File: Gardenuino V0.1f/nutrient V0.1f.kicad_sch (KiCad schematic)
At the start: 84 parts, among them J1 Conn_01x04_Male, J2 Conn_01x04_Female, J3 Conn_01x04_Male, J4 Conn_01x04_Male, J5 Conn_01x04_Female, J6 Conn_01x04_Male, J7 Conn_01x03_Male, J8 Conn_01x03_Male, P1 SolderJumper_2_Open, P2 SolderJumper_2_Bridged, P3 SolderJumper_2_Bridged, Q1 Q_NMOS_DGS, Q10 Q_NMOS_DGS, Q2 Q_NMOS_DGS, Q3 Q_NMOS_DGS, Q4 Q_NMOS_DGS, Q5 Q_NMOS_DGS, Q6 Q_NMOS_DGS, Q7 Q_NMOS_DGS, Q8 2N3904, U1 23LC512, U2 DS1307+, Y1 Crystal_Small

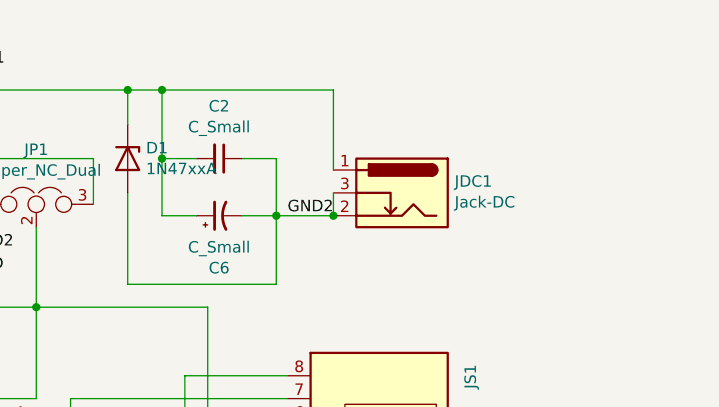
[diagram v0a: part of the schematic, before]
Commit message: SpectDrone development
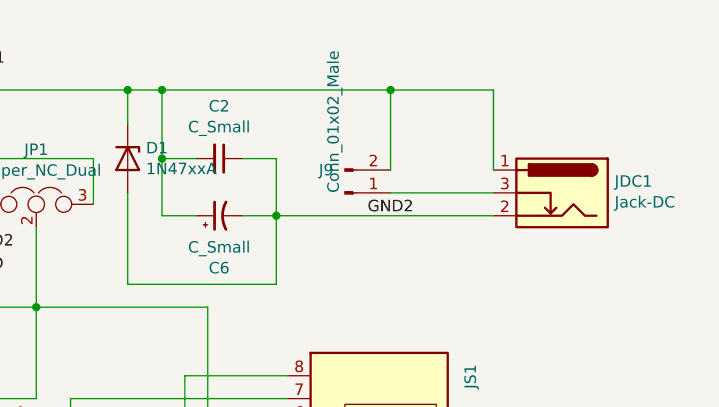
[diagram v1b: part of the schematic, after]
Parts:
- added J9: Conn_01x02_Male, Connector_PinHeader_2.54mm:PinHeader_1x02_P2.54mm_Vertical, symbol Connector:Conn_01x02_Male
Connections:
- net GND: no longer JDC1.3
- net VIN1: now also J9.2 (Pin_2)
- new net: J9.1 (Pin_1), JDC1.3
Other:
- moved on the sheet: JDC1
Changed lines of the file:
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@@
   (junction (at 267.97 110.49) (diameter 0) (color 0 0 0 0)
   )
+  (junction (at 250.19 17.78) (diameter 0) (color 0 0 0 0)
+  )
   (junction (at 227.33 125.73) (diameter 0) (color 0 0 0 0)
   )
@@
   )
   (junction (at 68.58 115.57) (diameter 0) (color 0 0 0 0)
-  )
-  (junction (at 243.84 31.75) (diameter 0) (color 0 0 0 0)
   )
   (junction (at 83.82 113.03) (diameter 0) (color 0 0 0 0)
@@
     (stroke (width 0) (type default) (color 0 0 0 0))
   )
+  (wire (pts (xy 237.49 31.75) (xy 261.62 31.75))
+    (stroke (width 0) (type default) (color 0 0 0 0))
+  )
   (wire (pts (xy 104.14 157.48) (xy 134.62 157.48))
     (stroke (width 0) (type default) (color 0 0 0 0))
@@
     (stroke (width 0) (type default) (color 0 0 0 0))
   )
-  (wire (pts (xy 243.84 31.75) (xy 237.49 31.75))
-    (stroke (width 0) (type default) (color 0 0 0 0))
-  )
   (wire (pts (xy 273.05 139.7) (xy 278.13 139.7))
     (stroke (width 0) (type default) (color 0 0 0 0))
@@
     (stroke (width 0) (type default) (color 0 0 0 0))
   )
-  (wire (pts (xy 224.79 17.78) (xy 243.84 17.78))
+  (wire (pts (xy 224.79 17.78) (xy 250.19 17.78))
     (stroke (width 0) (type default) (color 0 0 0 0))
   )
@@
     (stroke (width 0) (type default) (color 0 0 0 0))
   )
-  (wire (pts (xy 243.84 17.78) (xy 243.84 26.67))
+  (wire (pts (xy 261.62 17.78) (xy 261.62 26.67))
     (stroke (width 0) (type default) (color 0 0 0 0))
   )
@@
     (stroke (width 0) (type default) (color 0 0 0 0))
   )
+  (wire (pts (xy 250.19 29.21) (xy 261.62 29.21))
+    (stroke (width 0) (type default) (color 0 0 0 0))
+  )
   (wire (pts (xy 146.685 154.305) (xy 146.685 155.575))
     (stroke (width 0) (type default) (color 0 0 0 0))
@@
     (stroke (width 0) (type default) (color 0 0 0 0))
   )
-  (wire (pts (xy 243.84 29.21) (xy 243.84 31.75))
-    (stroke (width 0) (type default) (color 0 0 0 0))
-  )
   (wire (pts (xy 241.3 115.57) (xy 241.3 116.84))
     (stroke (width 0) (type default) (color 0 0 0 0))
@@
     (stroke (width 0) (type default) (color 0 0 0 0))
   )
+  (wire (pts (xy 250.19 17.78) (xy 261.62 17.78))
+    (stroke (width 0) (type default) (color 0 0 0 0))
+  )
   (wire (pts (xy 134.62 133.35) (xy 138.43 133.35))
     (stroke (width 0) (type default) (color 0 0 0 0))
@@
     (stroke (width 0) (type default) (color 0 0 0 0))
   )
+  (wire (pts (xy 250.19 17.78) (xy 250.19 26.67))
+    (stroke (width 0) (type default) (color 0 0 0 0))
+  )
   (wire (pts (xy 168.91 142.24) (xy 168.91 144.78))
     (stroke (width 0) (type default) (color 0 0 0 0))
@@
     (effects (font (size 1.27 1.27)) (justify left bottom))
   )
-  (label "GND2" (at 243.84 31.75 180)
+  (label "GND2" (at 252.73 31.75 180)
     (effects (font (size 1.27 1.27)) (justify right bottom))
   )
@@
     (pin "2")
   )
-  (symbol (lib_id "Connector:Barrel_Jack_Switch") (at 251.46 29.21 0) (mirror y) (unit 1)
-    (in_bom yes) (on_board yes)
-    (property "Reference" "JDC1" (id 0) (at 257.302 27.94 0)
+  (symbol (lib_id "Connector:Barrel_Jack_Switch") (at 269.24 29.21 0) (mirror y) (unit 1)
+    (in_bom yes) (on_board yes)
+    (property "Reference" "JDC1" (id 0) (at 275.082 27.94 0)
       (effects (font (size 1.27 1.27)) (justify right))
     )
-    (property "Value" "Jack-DC" (id 1) (at 257.302 30.2514 0)
+    (property "Value" "Jack-DC" (id 1) (at 275.082 30.2514 0)
       (effects (font (size 1.27 1.27)) (justify right))
     )
-    (property "Footprint" "Connector_BarrelJack:BarrelJack_Horizontal" (id 2) (at 250.19 30.226 0)
-      (effects (font (size 1.27 1.27)) hide)
-    )
-    (property "Datasheet" "~" (id 3) (at 250.19 30.226 0)
+    (property "Footprint" "Connector_BarrelJack:BarrelJack_Horizontal" (id 2) (at 267.97 30.226 0)
+      (effects (font (size 1.27 1.27)) hide)
+    )
+    (property "Datasheet" "~" (id 3) (at 267.97 30.226 0)
       (effects (font (size 1.27 1.27)) hide)
     )
@@
     (pin "2")
   )
+  (symbol (lib_id "Connector:Conn_01x02_Male") (at 245.11 29.21 0) (mirror x) (unit 1)
+    (in_bom yes) (on_board yes)
+    (property "Reference" "J9" (id 0) (at 243.84 26.6699 0)
+      (effects (font (size 1.27 1.27)) (justify right))
+    )
+    (property "Value" "Conn_01x02_Male" (id 1) (at 243.84 29.2099 90)
+      (effects (font (size 1.27 1.27)) (justify right))
+    )
+    (property "Footprint" "Connector_PinHeader_2.54mm:PinHeader_1x02_P2.54mm_Vertical" (id 2) (at 245.11 29.21 0)
+      (effects (font (size 1.27 1.27)) hide)
+    )
+    (property "Datasheet" "~" (id 3) (at 245.11 29.21 0)
+      (effects (font (size 1.27 1.27)) hide)
+    )
+    (pin "1")
+    (pin "2")
+  )
   (symbol (lib_id "Device:R") (at 93.345 33.655 180) (unit 1)
     (in_bom yes) (on_board yes)
@@
       (reference "J8") (unit 1) (value "Conn_01x03_Male") (footprint "Connector_JST:JST_EH_S3B-EH_1x03_P2.50mm_Horizontal")
     )
+    (path "/6c1a8a3c-f787-40e4-8cd3-77048eeb28fc"
+      (reference "J9") (unit 1) (value "Conn_01x02_Male") (footprint "Connector_PinHeader_2.54mm:PinHeader_1x02_P2.54mm_Vertical")
+    )
     (path "/00000000-0000-0000-0000-000062f67074"
